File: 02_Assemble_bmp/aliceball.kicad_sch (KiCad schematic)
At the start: 192 parts, among them J1 Conn_01x02, J10 Conn_01x01, J11 Conn_01x01, J12 Conn_01x01, J13 Conn_01x01, J14 Conn_01x01, J15 Conn_01x01, J16 Conn_01x01, J17 Conn_01x01, J18 Conn_02x04_Odd_Even, J2 Conn_01x01, J3 Conn_01x01, J4 Conn_01x01, J5 Conn_01x01, J6 Conn_01x01, J7 Conn_01x01, J8 Conn_01x01, J9 Conn_01x01, SW1 SW_PUSH, SW10 SW_PUSH, SW11 SW_PUSH, SW12 SW_PUSH, SW13 SW_PUSH, SW14 SW_PUSH, SW15 SW_PUSH, SW16 SW_PUSH, SW17 SW_PUSH, SW18 SW_PUSH, SW19 SW_PUSH, SW2 SW_PUSH, SW20 SW_PUSH, SW21 SW_PUSH, SW22 SW_PUSH, SW23 SW_PUSH, SW24 SW_PUSH, SW24_2 SW_PUSH, SW25 RotaryEncoder_Switch, SW26 SW_PUSH, SW27 SW_PUSH, SW28 SW_PUSH, SW29 SW_PUSH, SW3 SW_PUSH, SW30 SW_PUSH, SW31 SW_PUSH, SW32 SW_PUSH, SW33 SW_PUSH, SW34 SW_PUSH, SW35 SW_PUSH, SW36 SW_PUSH, SW37 SW_PUSH, SW38 SW_PUSH, SW39 SW_PUSH, SW4 SW_PUSH, SW40 SW_PUSH, SW41 SW_PUSH, SW42 SW_PUSH, SW43 SW_PUSH, SW44 SW_PUSH, SW45 SW_PUSH, SW46 SW_PUSH, SW47 SW_PUSH, SW48 SW_PUSH, SW49 SW_PUSH, SW5 SW_PUSH, SW6 SW_PUSH, SW7 SW_PUSH, SW8 SW_PUSH, SW9 SW_PUSH, U1 BLEMicroPro

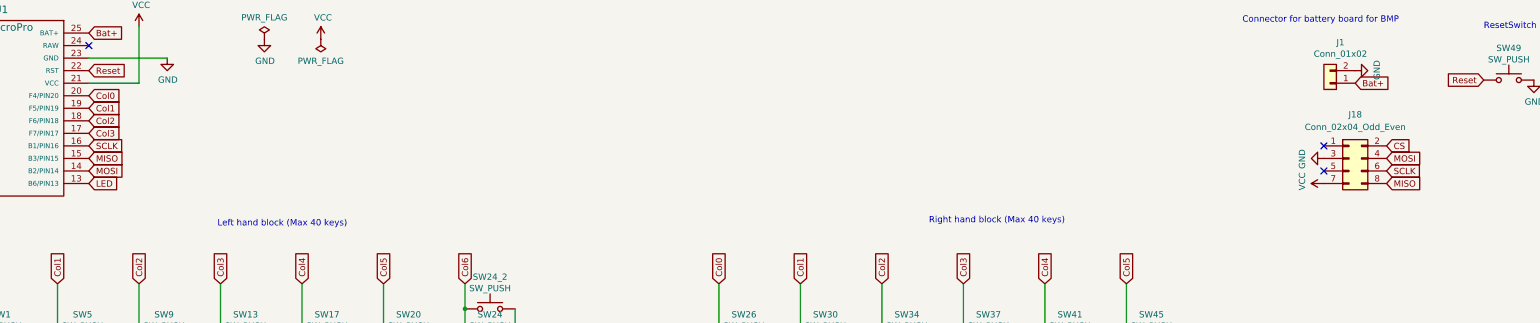
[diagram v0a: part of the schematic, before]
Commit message: rev 0.2
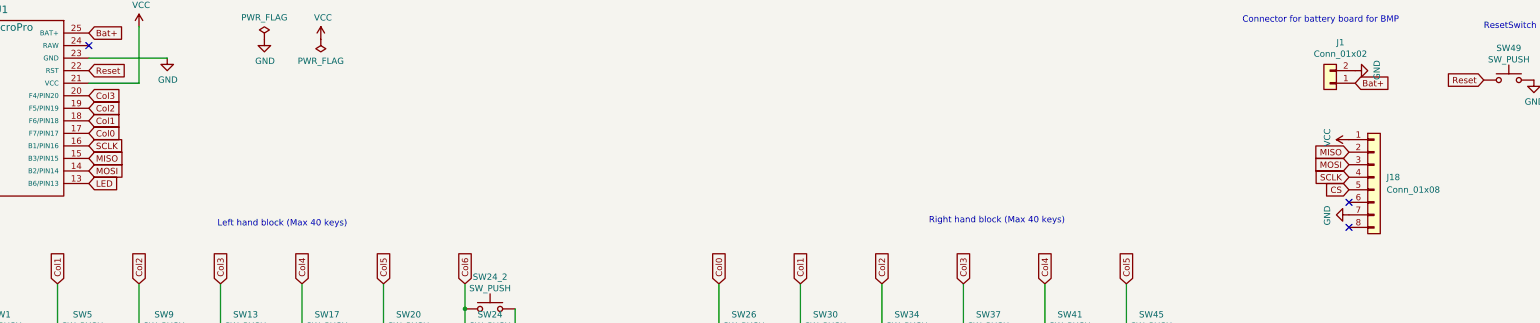
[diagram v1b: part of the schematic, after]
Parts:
- removed J18: Conn_02x04_Odd_Even, kbd_Parts:ADNS-9800-module, symbol Connector_Generic:Conn_02x04_Odd_Even
- added J18: Conn_01x08, kbd_Parts:PMW3389_board, symbol Connector_Generic:Conn_01x08
- D1, D10, D11, D12, D13, D14, D15, D16, D17, D18, D19, D2, D20, D21, D22, D23, D24, D25, D26, D27, D28, D29, D3, D30, D31, D32, D33, D34, D35, D36, D37, D38, D39, D4, D40, D41, D42, D43, D44, D45, D46, D47, D48, D5, D6, D7, D8, D9: footprint kbd_Parts:Diode_TH_SMD -> kbd_Parts:Diode_SMD
- H1, H10, H11, H12, H13, H14, H15, H16, H2, H3, H4, H5, H6, H7, H8, H9: footprint MountingHole:MountingHole_2.2mm_M2 -> kbd_Hole:m2_Screw_Hole
- L1, L10, L11, L12, L13, L14, L15, L16, L17, L18, L19, L2, L20, L21, L22, L23, L24, L25, L26, L27, L28, L29, L3, L30, L31, L32, L33, L34, L35, L36, L37, L38, L39, L4, L40, L41, L42, L43, L44, L45, L46, L47, L48, L49, L5, L50, L51, L52, L53, L54, L55, L56, L57, L58, L59, L6, L7, L8, L9: footprint kbd_Parts:LED_SK6812MINI-E_BL -> kbd_Parts:LED_SK6812MINI-E_BL_cut_silk
- SW1, SW10, SW11, SW13, SW14, SW15, SW17, SW18, SW19, SW20, SW21, SW22, SW23, SW24, SW26, SW27, SW28, SW29, SW30, SW31, SW32, SW34, SW35, SW36, SW37, SW38, SW39, SW4, SW42, SW43, SW44, SW46, SW47, SW48, SW5, SW6, SW7, SW8, SW9: footprint kbd_SW:CherryMX_Hotswap_1.0u -> kbd_SW:CherryMX_Hotswap_1u_no_silk
- SW12: footprint kbd_SW:CherryMX_Hotswap_1.0u -> kbd_SW:CherryMX_Hotswap_1.25u_no_silk
- SW16: footprint kbd_SW:CherryMX_Hotswap_2u -> kbd_SW:CherryMX_Hotswap_1.75u_no_silk
- SW2: footprint kbd_SW:CherryMX_Hotswap_1.25u -> kbd_SW:CherryMX_Hotswap_1.25u_no_silk
- SW3: footprint kbd_SW:CherryMX_Hotswap_1.75u -> kbd_SW:CherryMX_Hotswap_1.75u_no_silk
- SW33: footprint kbd_SW:CherryMX_Hotswap_2u -> kbd_SW:CherryMX_Hotswap_1.5u_no_silk
- SW40: footprint kbd_SW:CherryMX_Hotswap_1.0u -> kbd_SW:CherryMX_Hotswap_1.5u_no_silk
- SW41: footprint kbd_SW:CherryMX_Hotswap_1.0u -> kbd_SW:CherryMX_Hotswap_1u_Small1_no_silk
- SW45: footprint kbd_SW:CherryMX_Hotswap_1.5u -> kbd_SW:CherryMX_Hotswap_1.5u_no_silk
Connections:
- net CS: now also J18.5 (Pin_5)
- net Col0: now also U1.17 (F7/PIN17); no longer U1.20 (F4/PIN20)
- net Col1: now also U1.18 (F6/PIN18); no longer U1.19 (F5/PIN19)
- net Col2: now also U1.19 (F5/PIN19); no longer U1.18 (F6/PIN18)
- net Col3: now also U1.20 (F4/PIN20); no longer U1.17 (F7/PIN17)
- net GND: now also J18.7 (Pin_7)
- net MISO: now also J18.2 (Pin_2)
- net MOSI: now also J18.3 (Pin_3)
- net SCLK: now also J18.4 (Pin_4)
- net VCC: now also J18.1 (Pin_1)
